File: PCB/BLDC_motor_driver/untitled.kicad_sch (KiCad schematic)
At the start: 18 parts, among them J5 PHASE_A, Q8 CSD18533Q5A, Q9 CSD18533Q5A, U1 INA240A2D, U3 IR2104, U4 INA240A3D, U9 INA240A1D

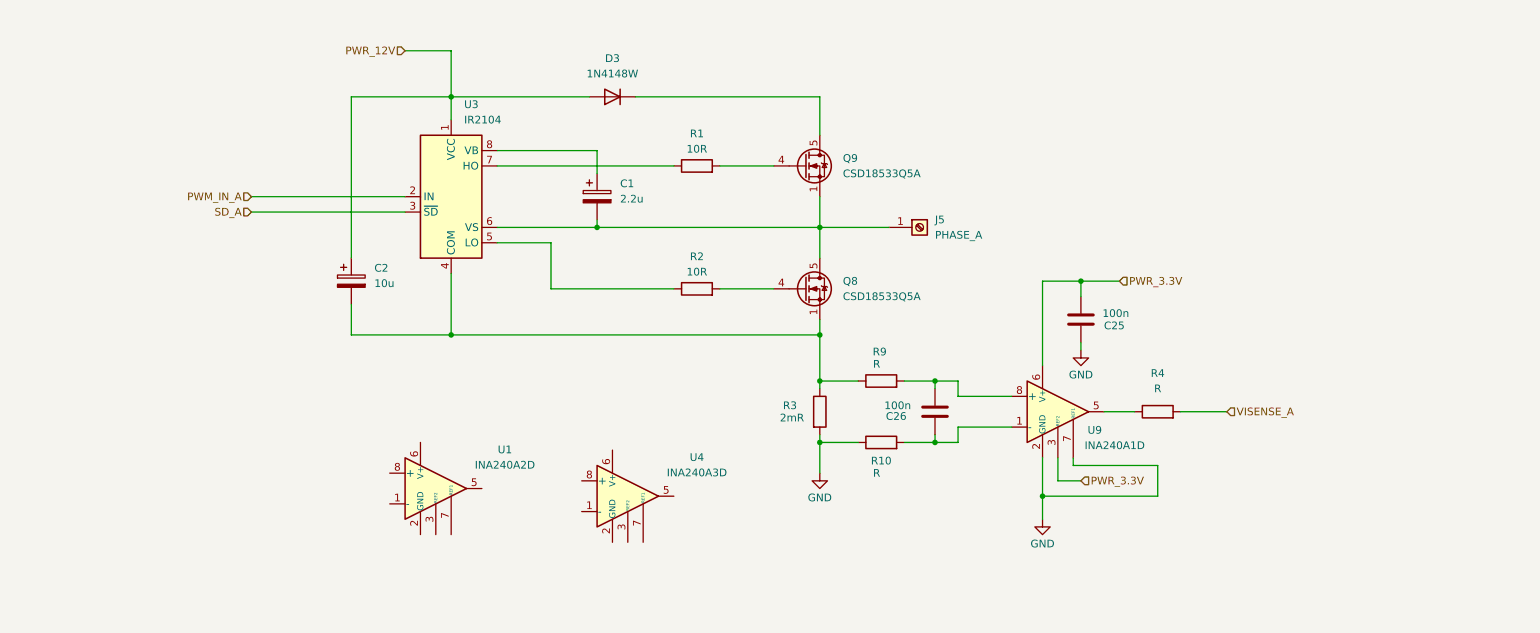
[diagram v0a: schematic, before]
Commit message: PCB v2 progress...
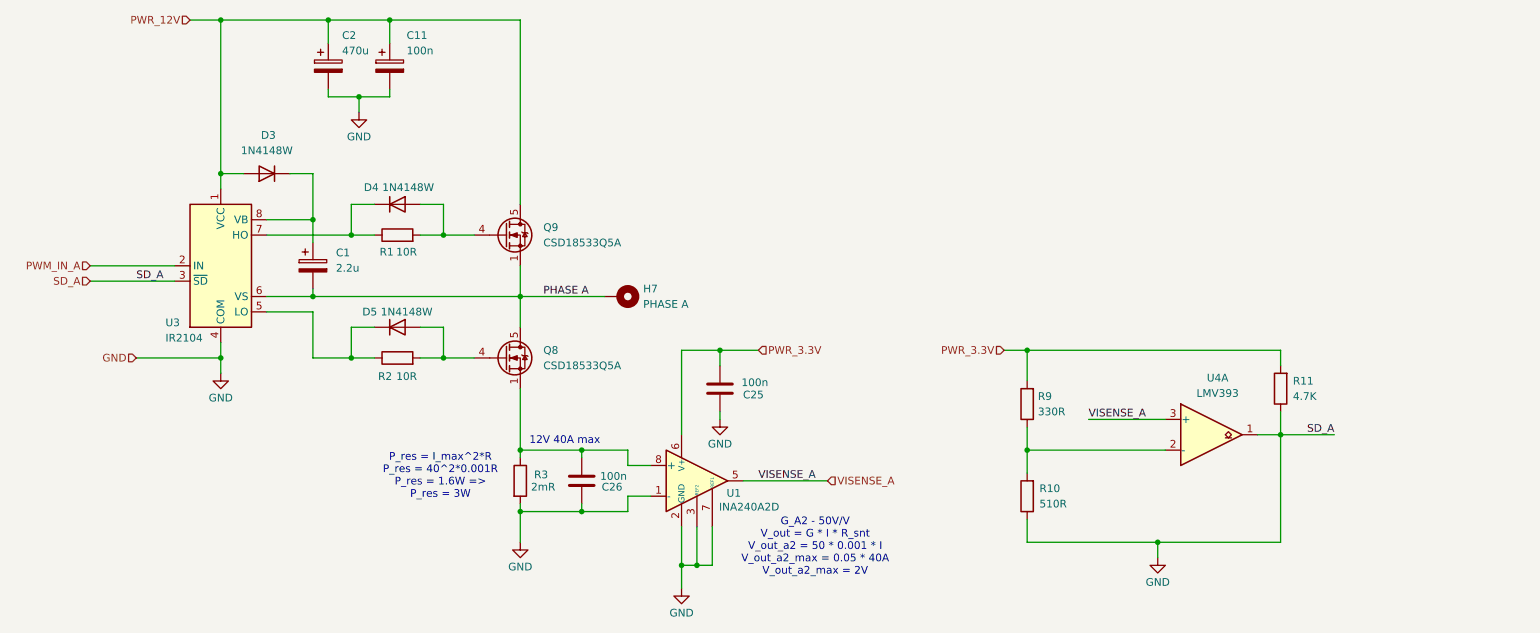
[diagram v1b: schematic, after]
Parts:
- removed J5: PHASE_A, TerminalBlock_MetzConnect:TerminalBlock_MetzConnect_360410_1x01_Horizontal_ScrewM3.0, symbol Connector:Screw_Terminal_01x01
- removed R4: R, symbol Device:R
- removed U4: INA240A3D, Package_SO:SOIC-8_3.9x4.9mm_P1.27mm, symbol Amplifier_Current:INA240A3D
- removed U9: INA240A1D, Package_SO:SOIC-8_3.9x4.9mm_P1.27mm, symbol Amplifier_Current:INA240A1D
- added C11: 100n, Capacitor_Tantalum_SMD:CP_EIA-2012-12_Kemet-R, symbol Device:C_Polarized
- added D4, D5: 1N4148W, Diode_SMD:D_SOD-123, symbol Diode:1N4148W
- added H7: PHASE A, MountingHole:MountingHole_2.2mm_M2_Pad_TopBottom, symbol Mechanical:MountingHole_Pad
- added R11: 4.7K, Resistor_SMD:R_0603_1608Metric, symbol Device:R
- added U4: LMV393, Package_SO:VSSOP-8_2.3x2mm_P0.5mm, symbol Comparator:LMV393
- C1: footprint Capacitor_Tantalum_SMD:CP_EIA-2012-15_AVX-P -> Capacitor_Tantalum_SMD:CP_EIA-2012-12_Kemet-R
- C2: value 10u -> 470u
- R10: value R -> 510R; footprint (none) -> Resistor_SMD:R_0603_1608Metric
- R9: value R -> 330R; footprint (none) -> Resistor_SMD:R_0603_1608Metric
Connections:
- net SD_A is gone; now on net GND: U3.3 (~{SD})
- net GND: now also C2.2, C26.2, U1.1 (-), U1.2 (GND), U1.3 (REF2), U1.4 (GND), U1.7 (REF1), U3.4 (COM), C11.2, R11.1, U4.1
- net PWR_12V: now also Q9.5 (D), C11.1
- net PWR_3.3V: now also R9.2, U1.6 (V+), R11.2
- net VISENSE_A: now also U1.5, U4.3 (+)
- net at R10.2: now also R9.1, U4.2 (-); no longer C26.2
- net at C26.1: now also Q8.1 (S), Q8.2 (S), Q8.3 (S), R3.1, U1.8 (+); no longer R9.2
- net at R2.1, U3.5 (LO): now also D5.1 (K)
- net PHASE A: now reaches C1.2, Q8.5 (D), Q9.1 (S), Q9.2 (S), Q9.3 (S), U3.6 (VS)
- net PHASE A: now also H7.1
- net at R1.1, U3.7 (HO): now also D4.1 (K)
- net at C1.1, U3.8 (VB): now also D3.1 (K)
- net at Q8.4 (G), R2.2: now also D5.2 (A)
- net at Q9.4 (G), R1.2: now also D4.2 (A)
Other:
- note added: "12V 40A max"
- note added: "G_A2 - 50V/V V_out = G * I * R_snt V_out_a2 = 50 * 0.001 * I V_out_a2_max = 0.05 * 40A V_out_a2_max = 2V"
- note added: "P_res = I_max^2*R P_res = 40^2*0.001R P_res = 1.6W => P_res = 3W"
- moved on the sheet: C1, C2, C25, C26, D3, Q8, Q9, R1, R2, R3, U1, U3

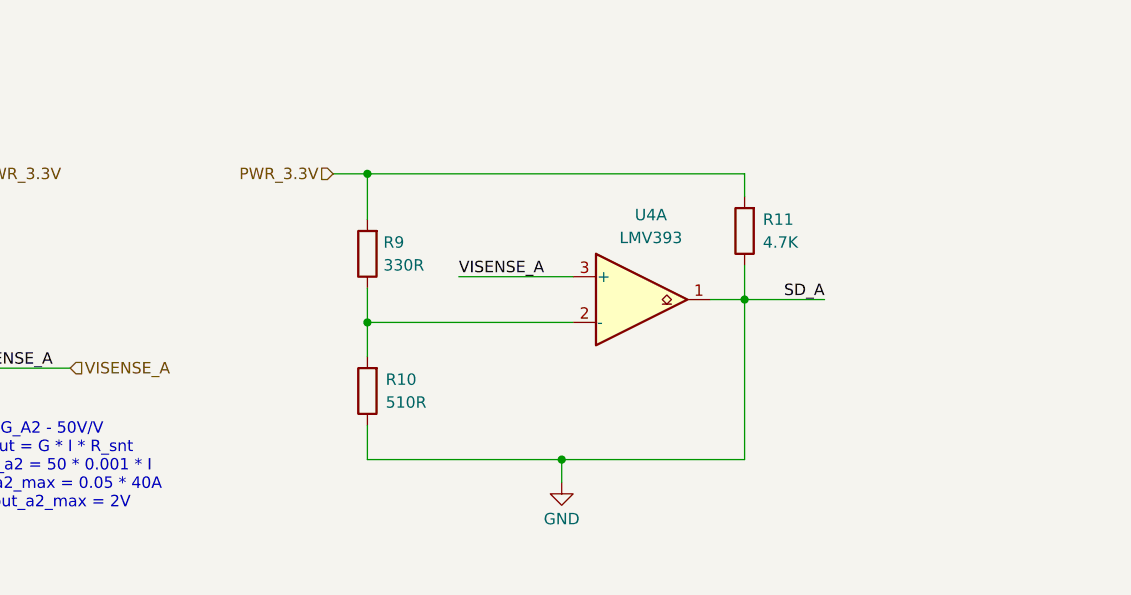
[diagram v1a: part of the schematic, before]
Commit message: Test driver layour finished... final touches
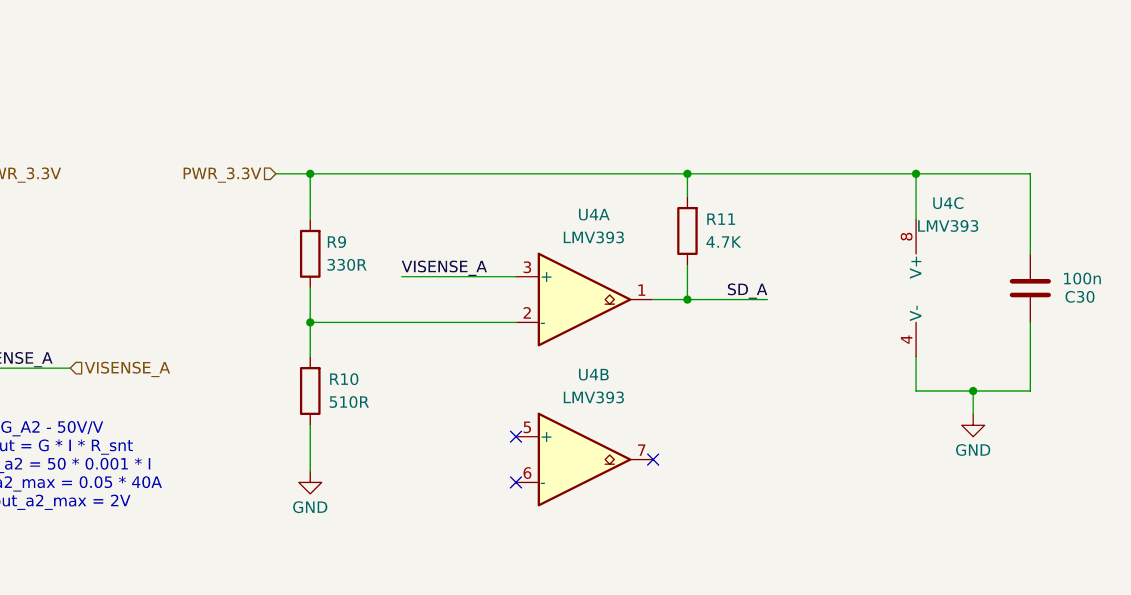
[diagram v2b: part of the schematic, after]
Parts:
- added C30: 100n, Capacitor_SMD:C_0402_1005Metric, symbol Device:C
- added unit 3 of U4
- added unit 2 of U4
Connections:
- net GND: now also C30.2, U4.4 (V-); no longer R11.1, U3.3 (~{SD}), U4.1
- net PWR_3.3V: now also C30.1, U4.8 (V+)
- new net SD_A: R11.1, U3.3 (~{SD}), U4.1
- no-connect marks 0 -> 3
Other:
- moved on the sheet: R10, R11, R9, U4A
